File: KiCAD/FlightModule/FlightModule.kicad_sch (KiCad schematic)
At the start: 13 parts

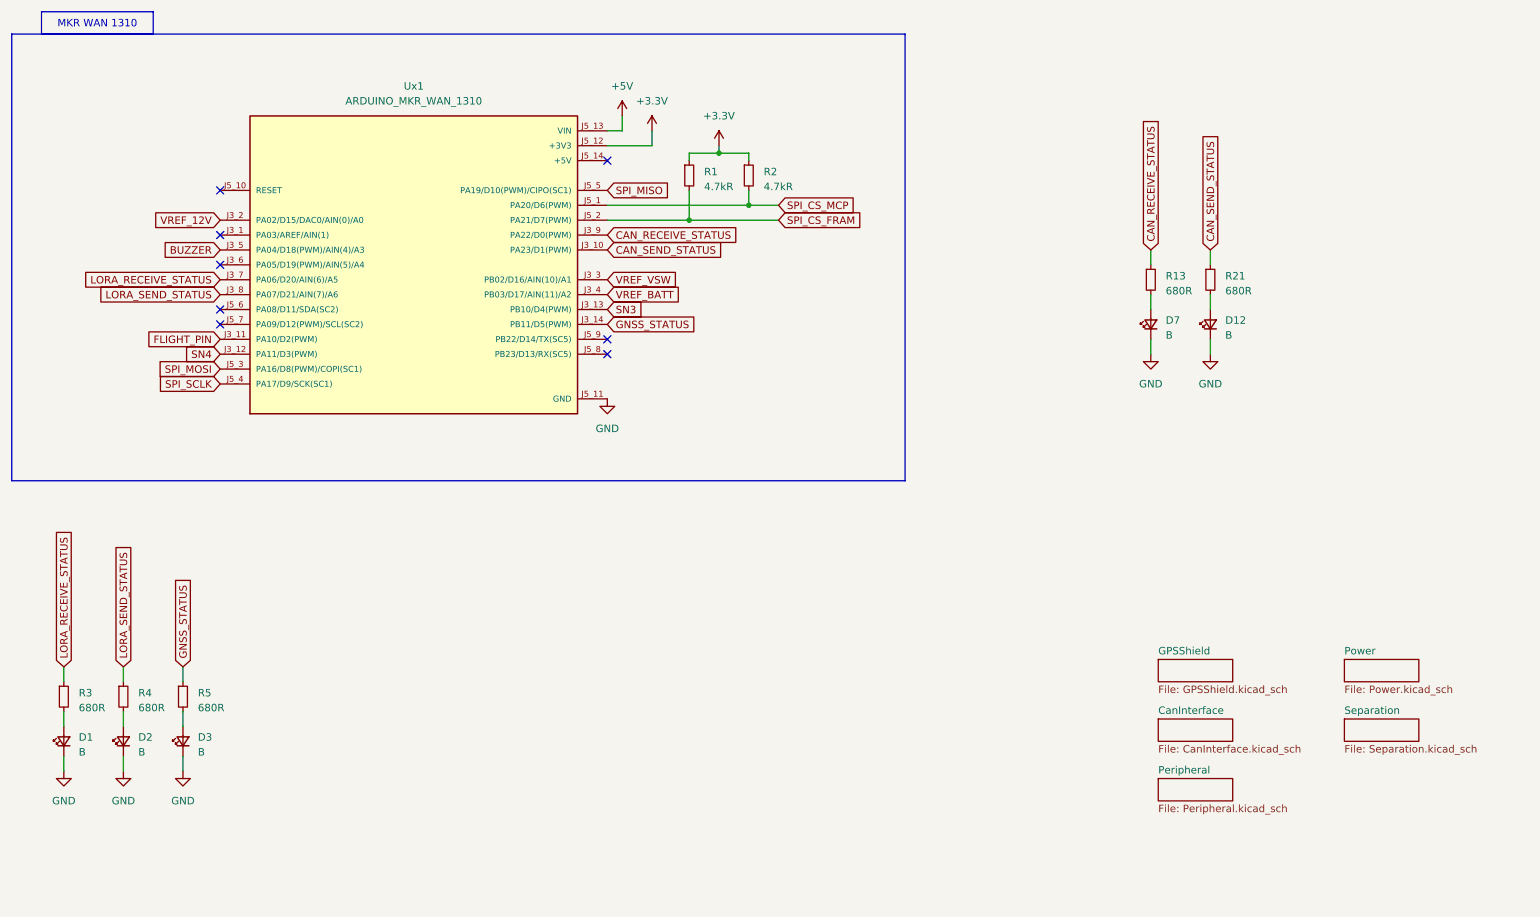
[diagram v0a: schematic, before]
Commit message: 回路図8割完成
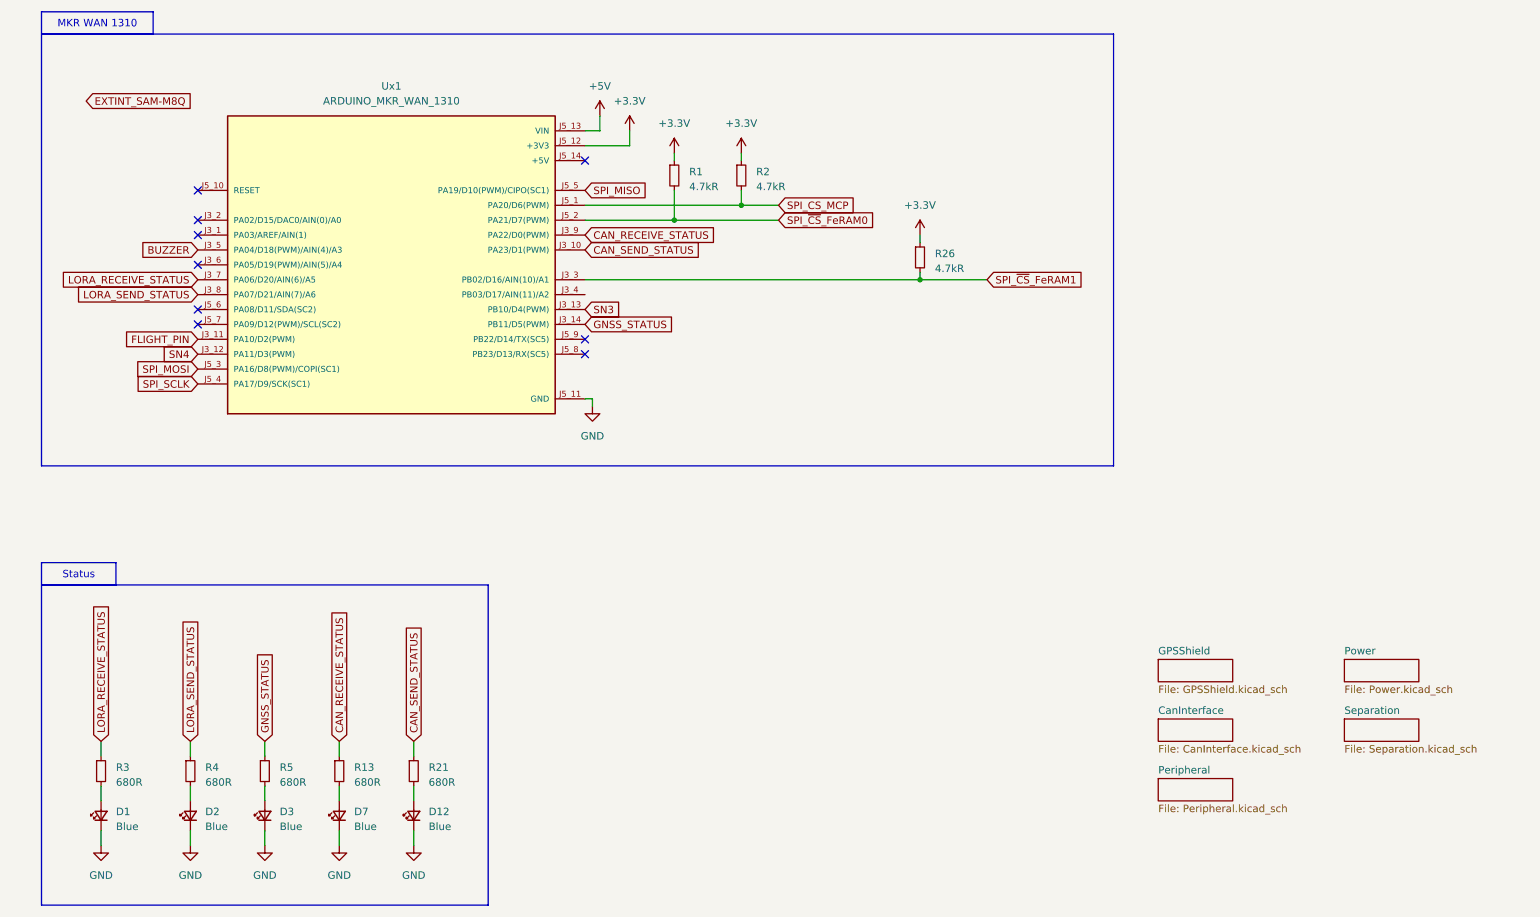
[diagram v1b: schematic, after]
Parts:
- added R26: 4.7kR, Resistor_SMD:R_0603_1608Metric_Pad0.98x0.95mm_HandSolder, symbol Device:R_Small
- D1, D12, D2, D3, D7: value B -> Blue
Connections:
- net +3.3V: now also R26.1
- net SPI_CS_FRAM renamed SPI_~{CS}_FeRAM0
- net VREF_12V: no longer names the net of Ux1.J3_2 (PA02/D15/DAC0/AIN(0)/A0)
- net VREF_BATT: no longer names the net of Ux1.J3_4 (PB03/D17/AIN(11)/A2)
- net VREF_VSW renamed SPI_~{CS}_FeRAM1
- net SPI_~{CS}_FeRAM1: now also R26.2
- no-connect marks 8 -> 9
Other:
- moved on the sheet: D1, D12, D2, D3, D7, R1, R13, R2, R21, R3, R4, R5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

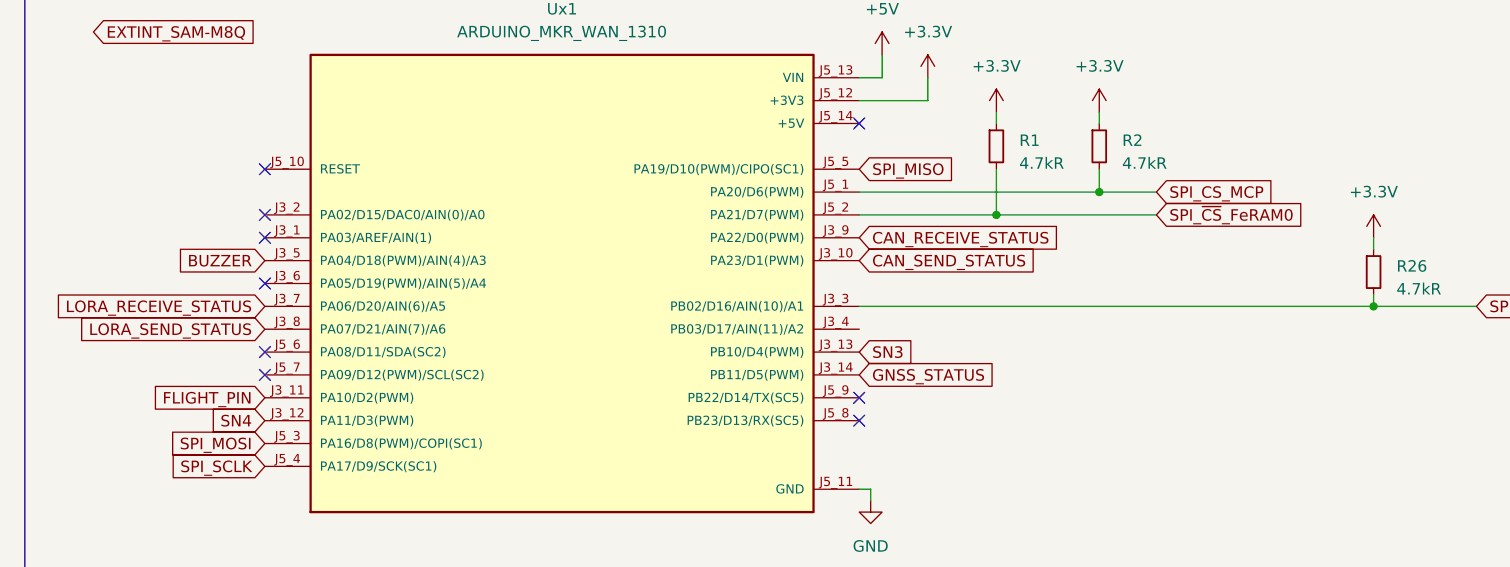
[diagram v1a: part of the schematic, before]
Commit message: 配線8割り終わり．次の作業....
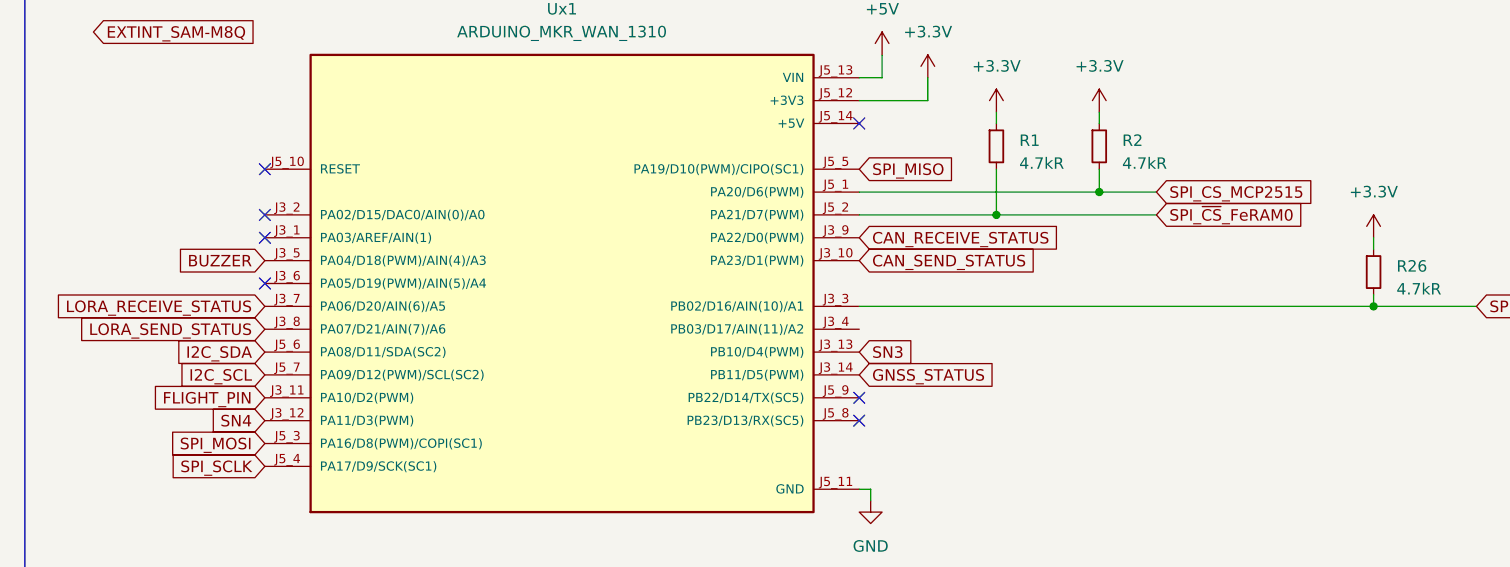
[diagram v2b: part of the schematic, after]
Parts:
- Ux1: footprint ARDUINO_MKR_WAN_1310:BOARD_ARDUINO_MKR_WAN_1310 -> TSRP_Arduino:BOARD_ARDUINO_MKR_WAN_1310
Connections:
- net I2C_SDA: now reaches Ux1.J5_6 (PA08/D11/SDA(SC2))
- net I2C_SCL: now reaches Ux1.J5_7 (PA09/D12(PWM)/SCL(SC2))
- net SPI_CS_MCP renamed SPI_CS_MCP2515
- no-connect marks 9 -> 7
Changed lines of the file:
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@@
 		(at 118.11 80.01)
 	)
-	(no_connect
-		(at 52.07 72.39)
-	)
-	(no_connect
-		(at 52.07 74.93)
-	)
 	(wire
 		(pts
@@
 		)
 	)
-	(global_label "SPI_CS_MCP"
+	(global_label "SPI_CS_MCP2515"
 		(shape input)
 		(at 151.13 54.61 0)
@@
 		)
 		(property "Intersheetrefs" "${INTERSHEET_REFS}"
-			(at 165.6056 54.61 0)
+			(at 170.4436 54.61 0)
 			(effects
 				(font
@@
 		)
 	)
+	(global_label "I2C_SDA"
+		(shape input)
+		(at 52.07 72.39 180)
+		(fields_autoplaced yes)
+		(effects
+			(font
+				(size 1.27 1.27)
+			)
+			(justify right)
+		)
+		(property "Intersheetrefs" "${INTERSHEET_REFS}"
+			(at 41.4648 72.39 0)
+			(effects
+				(font
+					(size 1.27 1.27)
+				)
+				(justify right)
+				(hide yes)
+			)
+		)
+	)
 	(global_label "CAN_SEND_STATUS"
 		(shape input)
@@
 		)
 	)
+	(global_label "I2C_SCL"
+		(shape input)
+		(at 52.07 74.93 180)
+		(fields_autoplaced yes)
+		(effects
+			(font
+				(size 1.27 1.27)
+			)
+			(justify right)
+		)
+		(property "Intersheetrefs" "${INTERSHEET_REFS}"
+			(at 41.5253 74.93 0)
+			(effects
+				(font
+					(size 1.27 1.27)
+				)
+				(justify right)
+				(hide yes)
+			)
+		)
+	)
 	(global_label "CAN_RECEIVE_STATUS"
 		(shape input)
@@
 				(justify left)
 				(hide yes)
+			)
+		)
+	)
+	(symbol
+		(lib_id "power:+3.3V")
+		(at 125.73 41.91 0)
+		(unit 1)
+		(exclude_from_sim no)
+		(in_bom yes)
+		(on_board yes)
+		(dnp no)
+		(fields_autoplaced yes)
+		(property "Reference" "#PWR051"
+			(at 125.73 45.72 0)
+			(effects
+				(font
+					(size 1.27 1.27)
+				)
+				(hide yes)
+			)
+		)
+		(property "Value" "+3.3V"
+			(at 125.73 36.83 0)
+			(effects
+				(font
+					(size 1.27 1.27)
+				)
+			)
+		)
+		(property "Footprint" ""
+			(at 125.73 41.91 0)
+			(effects
+				(font
+					(size 1.27 1.27)
+				)
+				(hide yes)
+			)
+		)
+		(property "Datasheet" ""
+			(at 125.73 41.91 0)
+			(effects
+				(font
+					(size 1.27 1.27)
+				)
+				(hide yes)
+			)
+		)
+		(property "Description" "Power symbol creates a global label with name \"+3.3V\""
+			(at 125.73 41.91 0)
+			(effects
+				(font
+					(size 1.27 1.27)
+				)
+				(hide yes)
+			)
+		)
+		(pin "1"
+		)
+		(instances
+			(project "FlightModule"
+				(path "/3507137a-fdd7-4bc0-abe8-370b7c3b390e"
+					(reference "#PWR051")
+					(unit 1)
+				)
 			)
 		)
@@
 	(symbol
 		(lib_id "power:+3.3V")
-		(at 125.73 41.91 0)
-		(unit 1)
-		(exclude_from_sim no)
-		(in_bom yes)
-		(on_board yes)
-		(dnp no)
-		(fields_autoplaced yes)
-		(property "Reference" "#PWR06"
-			(at 125.73 45.72 0)
-			(effects
-				(font
-					(size 1.27 1.27)
-				)
-				(hide yes)
-			)
-		)
-		(property "Value" "+3.3V"
-			(at 125.73 36.83 0)
-			(effects
-				(font
-					(size 1.27 1.27)
-				)
-			)
-		)
-		(property "Footprint" ""
-			(at 125.73 41.91 0)
-			(effects
-				(font
-					(size 1.27 1.27)
-				)
-				(hide yes)
-			)
-		)
-		(property "Datasheet" ""
-			(at 125.73 41.91 0)
-			(effects
-				(font
-					(size 1.27 1.27)
-				)
-				(hide yes)
-			)
-		)
-		(property "Description" "Power symbol creates a global label with name \"+3.3V\""
-			(at 125.73 41.91 0)
-			(effects
-				(font
-					(size 1.27 1.27)
-				)
-				(hide yes)
-			)
-		)
-		(pin "1"
-		)
-		(instances
-			(project ""
-				(path "/3507137a-fdd7-4bc0-abe8-370b7c3b390e"
-					(reference "#PWR06")
-					(unit 1)
-				)
-			)
-		)
-	)
-	(symbol
-		(lib_id "power:+3.3V")
 		(at 133.35 45.72 0)
 		(unit 1)
@@
 			)
 		)
-		(property "Footprint" "ARDUINO_MKR_WAN_1310:BOARD_ARDUINO_MKR_WAN_1310"
+		(property "Footprint" "TSRP_Arduino:BOARD_ARDUINO_MKR_WAN_1310"
 			(at 85.09 64.77 0)
 			(effects
